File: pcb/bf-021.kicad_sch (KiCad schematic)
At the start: 12 parts, among them J1 M-BUS, U1 SCD40-D-R2

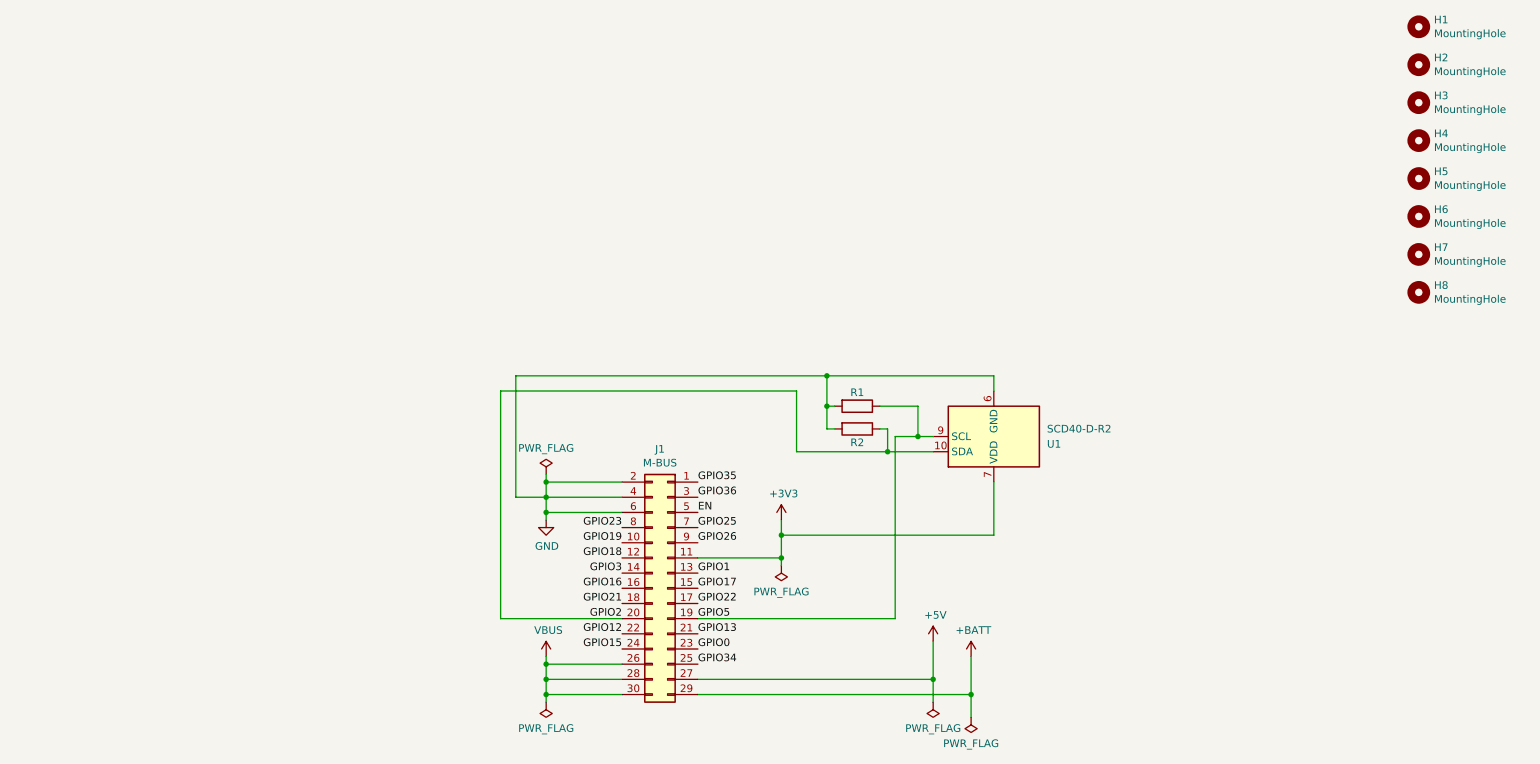
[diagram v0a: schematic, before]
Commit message: improved design
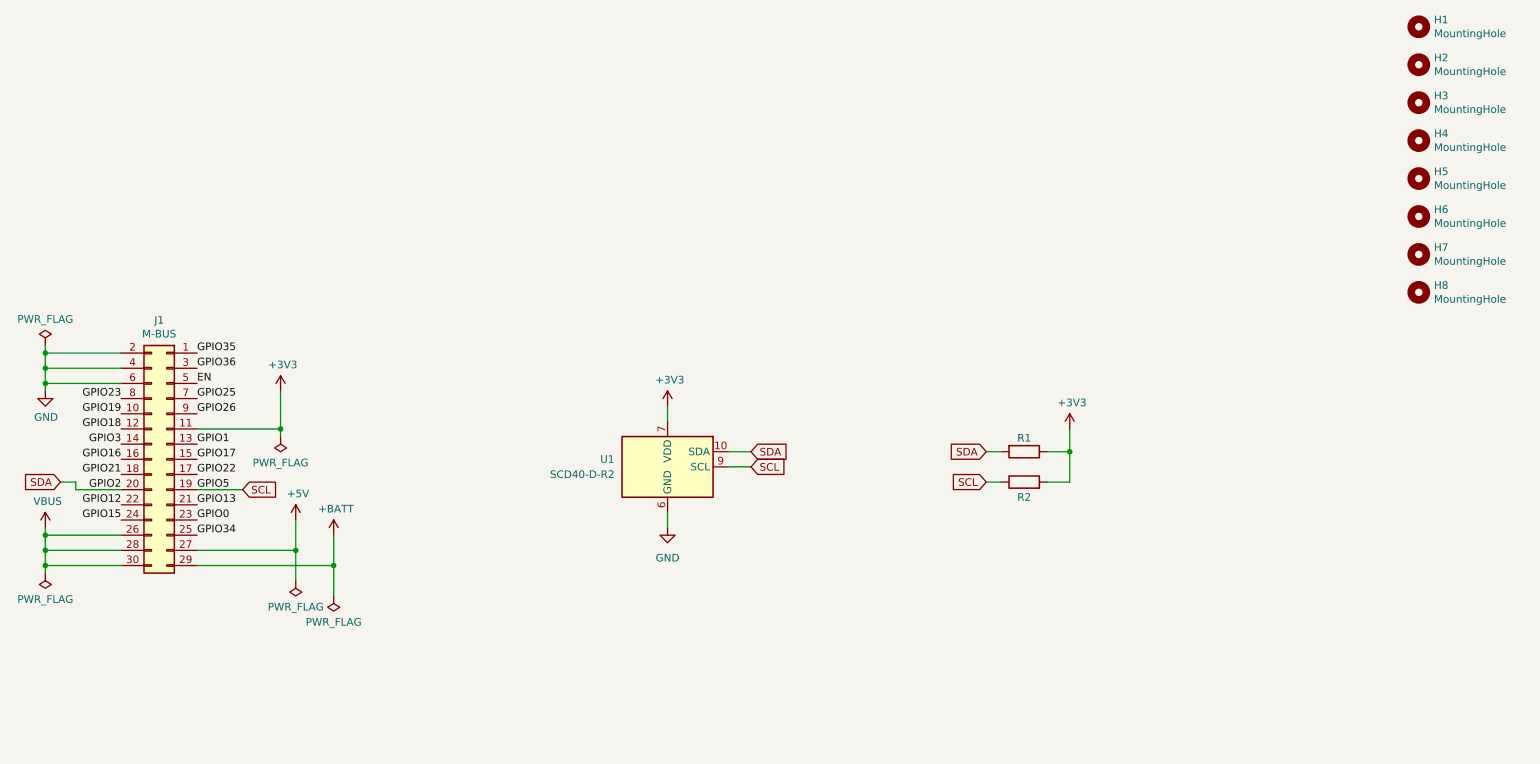
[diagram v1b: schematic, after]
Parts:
- R1, R2: value R -> 10k; footprint Resistor_THT:R_Axial_DIN0207_L6.3mm_D2.5mm_P7.62mm_Horizontal -> Resistor_SMD:R_0603_1608Metric_Pad0.98x0.95mm_HandSolder
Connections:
- net +3V3: now also R1.1, R2.2
- net GND: no longer R1.2, R2.2
- net GPIO2 renamed SDA
- net SDA: now also R1.2; no longer R2.1
- net GPIO5 renamed SCL
- net SCL: now also R2.1; no longer R1.1
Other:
- moved on the sheet: J1, R1, R2, U1
